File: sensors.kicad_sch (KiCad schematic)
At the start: 13 parts, among them J2 Conn_Coaxial, U14 ISM6HG256X, U18 LIS2MDL, U3 MS5607-02BA, U5 MAX-M10S

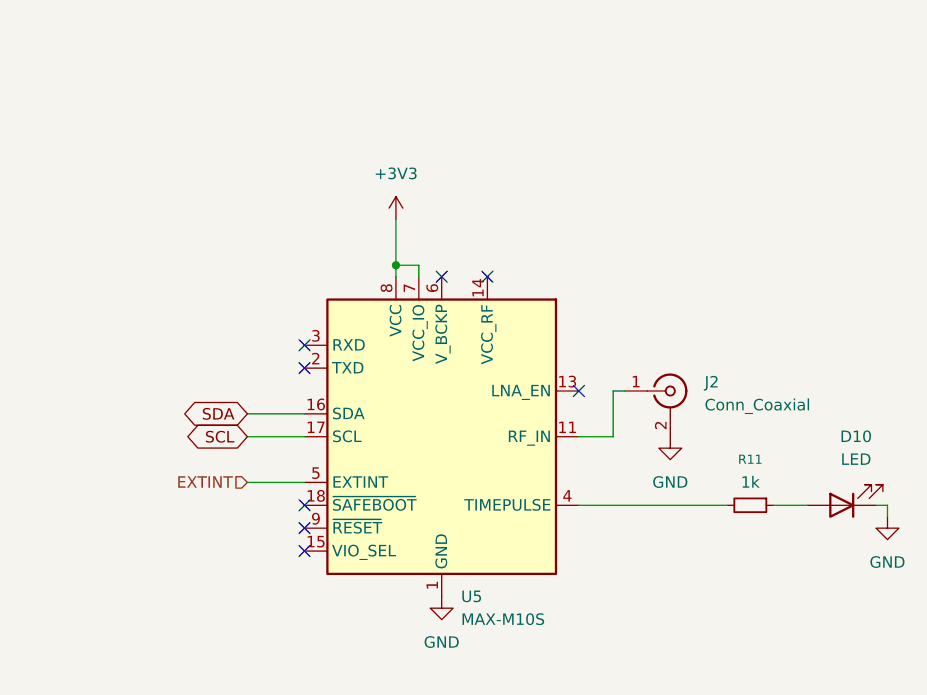
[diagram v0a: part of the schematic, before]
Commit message: remove unneeded stuff
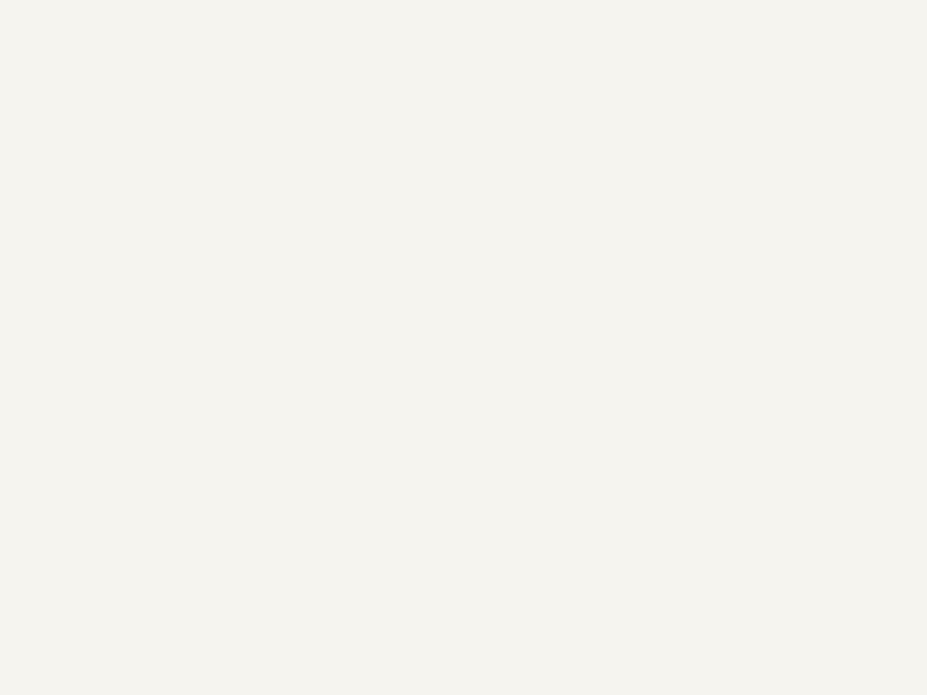
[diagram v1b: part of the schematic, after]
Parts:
- removed D10: LED, LED_SMD:LED_0805_2012Metric, symbol Device:LED
- removed J2: Conn_Coaxial, Connector_Coaxial:U.FL_Hirose_U.FL-R-SMT-1_Vertical, symbol Connector:Conn_Coaxial
- removed R11: 1k, Resistor_SMD:R_0402_1005Metric, symbol Device:R_Small
- removed U5: MAX-M10S, RF_GPS:ublox_MAX, symbol RF_GPS:MAX-M10S
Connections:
- no-connect marks 12 -> 4
